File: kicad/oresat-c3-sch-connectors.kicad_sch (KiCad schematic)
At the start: 15 parts, among them J1 Conn_02x26_Odd_Even, J2 Conn_02x26_Odd_Even, J7 2-1734592-0

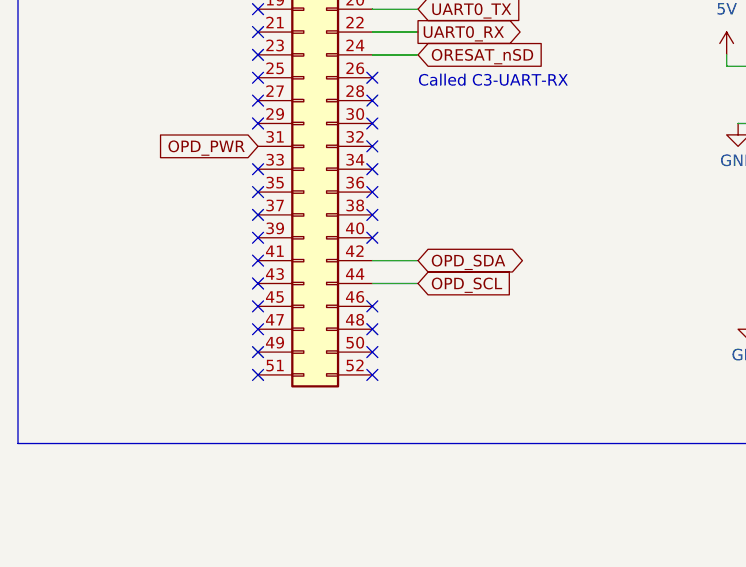
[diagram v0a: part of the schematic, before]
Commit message: Added I2C1 bus lines
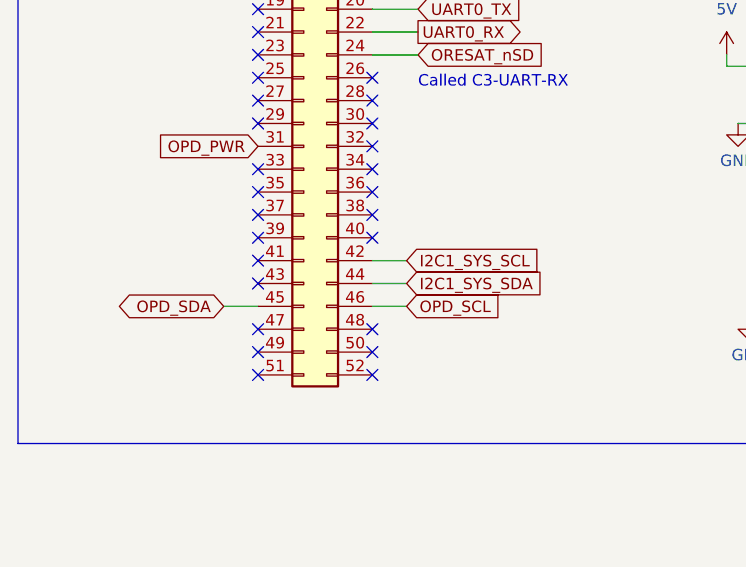
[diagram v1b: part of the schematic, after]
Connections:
- net OPD_SCL: now also J1.46 (Pin_46); no longer J1.44 (Pin_44)
- net OPD_SDA: now also J1.45 (Pin_45); no longer J1.42 (Pin_42)
- new net I2C1_SYS_SCL: J1.42 (Pin_42)
- new net I2C1_SYS_SDA: J1.44 (Pin_44)
- no-connect marks 92 -> 90
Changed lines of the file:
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@@
-	)
-	(no_connect
-		(at 113.03 113.03)
 	)
 	(no_connect
@@
 	)
 	(no_connect
-		(at 125.73 113.03)
-	)
-	(no_connect
 		(at 173.99 58.42)
 	)
@@
 	(wire
 		(pts
-			(xy 125.73 110.49) (xy 130.81 110.49)
-		)
-		(stroke
-			(width 0)
-			(type default)
-		)
-	)
-	(wire
-		(pts
 			(xy 275.59 101.6) (xy 273.05 101.6)
 		)
@@
 	(wire
 		(pts
-			(xy 125.73 107.95) (xy 130.81 107.95)
-		)
-		(stroke
-			(width 0)
-			(type default)
-		)
-	)
-	(wire
-		(pts
 			(xy 273.05 111.76) (xy 275.59 111.76)
 		)
@@
 	(wire
 		(pts
+			(xy 125.73 110.49) (xy 129.54 110.49)
+		)
+		(stroke
+			(width 0)
+			(type default)
+		)
+	)
+	(wire
+		(pts
 			(xy 262.89 130.81) (xy 262.89 134.62)
 		)
@@
 	(wire
 		(pts
+			(xy 125.73 113.03) (xy 129.54 113.03)
+		)
+		(stroke
+			(width 0)
+			(type default)
+		)
+	)
+	(wire
+		(pts
 			(xy 171.45 91.44) (xy 171.45 92.71)
 		)
@@
 	(wire
 		(pts
+			(xy 125.73 107.95) (xy 129.54 107.95)
+		)
+		(stroke
+			(width 0)
+			(type default)
+		)
+	)
+	(wire
+		(pts
 			(xy 166.37 92.71) (xy 171.45 92.71)
 		)
@@
 		(pts
 			(xy 167.64 114.3) (xy 173.99 114.3)
+		)
+		(stroke
+			(width 0)
+			(type default)
+		)
+	)
+	(wire
+		(pts
+			(xy 109.22 113.03) (xy 113.03 113.03)
 		)
 		(stroke
@@
 		)
 	)
+	(global_label "I2C1_SYS_SDA"
+		(shape input)
+		(at 129.54 110.49 0)
+		(fields_autoplaced yes)
+		(effects
+			(font
+				(size 1.27 1.27)
+			)
+			(justify left)
+		)
+		(property "Intersheetrefs" "${INTERSHEET_REFS}"
+			(at 145.8299 110.49 0)
+			(effects
+				(font
+					(size 1.27 1.27)
+				)
+				(justify left)
+			)
+		)
+	)
 	(global_label "OPD_SDA"
 		(shape bidirectional)
-		(at 130.81 107.95 0)
-		(fields_autoplaced yes)
-		(effects
-			(font
-				(size 1.27 1.27)
-			)
-			(justify left)
-		)
-		(property "Intersheetrefs" "${INTERSHEET_REFS}"
-			(at 143.3127 107.95 0)
-			(effects
-				(font
-					(size 1.27 1.27)
-				)
-				(justify left)
+		(at 109.22 113.03 180)
+		(fields_autoplaced yes)
+		(effects
+			(font
+				(size 1.27 1.27)
+			)
+			(justify right)
+		)
+		(property "Intersheetrefs" "${INTERSHEET_REFS}"
+			(at 96.7173 113.03 0)
+			(effects
+				(font
+					(size 1.27 1.27)
+				)
+				(justify right)
 			)
 		)
@@
 		)
 	)
+	(global_label "I2C1_SYS_SCL"
+		(shape input)
+		(at 129.54 107.95 0)
+		(fields_autoplaced yes)
+		(effects
+			(font
+				(size 1.27 1.27)
+			)
+			(justify left)
+		)
+		(property "Intersheetrefs" "${INTERSHEET_REFS}"
+			(at 145.7694 107.95 0)
+			(effects
+				(font
+					(size 1.27 1.27)
+				)
+				(justify left)
+			)
+		)
+	)
 	(global_label "USB_CLI_DM"
 		(shape bidirectional)
@@
 	(global_label "OPD_SCL"
 		(shape input)
-		(at 130.81 110.49 0)
-		(fields_autoplaced yes)
-		(effects
-			(font
-				(size 1.27 1.27)
-			)
-			(justify left)
-		)
-		(property "Intersheetrefs" "${INTERSHEET_REFS}"
-			(at 142.1409 110.49 0)
-			(effects
-				(font
+		(at 129.54 113.03 0)
+		(fields_autoplaced yes)
+		(effects
+			(font
+				(size 1.27 1.27)
+			)
+			(justify left)
+		)
+		(property "Intersheetrefs" "${INTERSHEET_REFS}"
+			(at 140.8709 113.03 0)
+			(effects
+				(font

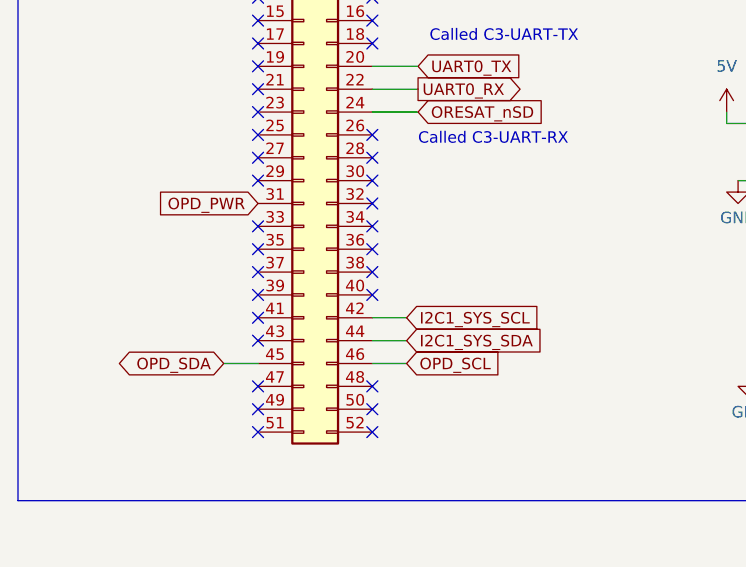
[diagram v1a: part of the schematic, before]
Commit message: Removed OPD and added LTC4300A to I2C1 bus
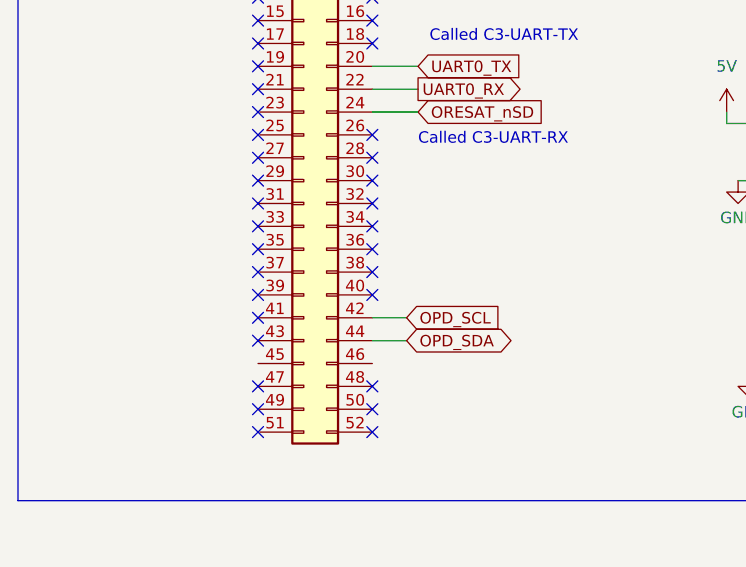
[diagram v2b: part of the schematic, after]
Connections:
- net I2C1_SYS_SCL is gone; now on net OPD_SCL: J1.42 (Pin_42)
- net I2C1_SYS_SDA is gone; now on net OPD_SDA: J1.44 (Pin_44)
- net OPD_SCL: no longer J1.46 (Pin_46)
- net OPD_SDA: no longer J1.45 (Pin_45)
- net OPD_PWR: no longer names the net of J1.31 (Pin_31)
- no-connect marks 90 -> 91
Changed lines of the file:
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@@
+	)
+	(no_connect
+		(at 113.03 95.25)
 	)
 	(no_connect
@@
 	(wire
 		(pts
+			(xy 262.89 130.81) (xy 262.89 134.62)
+		)
+		(stroke
+			(width 0)
+			(type default)
+		)
+	)
+	(wire
+		(pts
+			(xy 125.73 107.95) (xy 129.54 107.95)
+		)
+		(stroke
+			(width 0)
+			(type default)
+		)
+	)
+	(wire
+		(pts
+			(xy 274.32 130.81) (xy 262.89 130.81)
+		)
+		(stroke
+			(width 0)
+			(type default)
+		)
+	)
+	(wire
+		(pts
+			(xy 280.67 96.52) (xy 273.05 96.52)
+		)
+		(stroke
+			(width 0)
+			(type default)
+		)
+	)
+	(wire
+		(pts
+			(xy 279.4 73.66) (xy 280.67 73.66)
+		)
+		(stroke
+			(width 0)
+			(type default)
+		)
+	)
+	(wire
+		(pts
+			(xy 280.67 88.9) (xy 273.05 88.9)
+		)
+		(stroke
+			(width 0)
+			(type default)
+		)
+	)
+	(wire
+		(pts
 			(xy 125.73 110.49) (xy 129.54 110.49)
 		)
@@
 	(wire
 		(pts
-			(xy 262.89 130.81) (xy 262.89 134.62)
-		)
-		(stroke
-			(width 0)
-			(type default)
-		)
-	)
-	(wire
-		(pts
-			(xy 274.32 130.81) (xy 262.89 130.81)
-		)
-		(stroke
-			(width 0)
-			(type default)
-		)
-	)
-	(wire
-		(pts
-			(xy 280.67 96.52) (xy 273.05 96.52)
-		)
-		(stroke
-			(width 0)
-			(type default)
-		)
-	)
-	(wire
-		(pts
-			(xy 279.4 73.66) (xy 280.67 73.66)
-		)
-		(stroke
-			(width 0)
-			(type default)
-		)
-	)
-	(wire
-		(pts
-			(xy 280.67 88.9) (xy 273.05 88.9)
-		)
-		(stroke
-			(width 0)
-			(type default)
-		)
-	)
-	(wire
-		(pts
 			(xy 186.69 86.36) (xy 194.31 86.36)
 		)
@@
 	(wire
 		(pts
-			(xy 125.73 113.03) (xy 129.54 113.03)
-		)
-		(stroke
-			(width 0)
-			(type default)
-		)
-	)
-	(wire
-		(pts
 			(xy 171.45 91.44) (xy 171.45 92.71)
 		)
@@
 	(wire
 		(pts
-			(xy 125.73 107.95) (xy 129.54 107.95)
-		)
-		(stroke
-			(width 0)
-			(type default)
-		)
-	)
-	(wire
-		(pts
 			(xy 166.37 92.71) (xy 171.45 92.71)
 		)
@@
 		(pts
 			(xy 167.64 114.3) (xy 173.99 114.3)
-		)
-		(stroke
-			(width 0)
-			(type default)
-		)
-	)
-	(wire
-		(pts
-			(xy 109.22 113.03) (xy 113.03 113.03)
 		)
 		(stroke
@@
 		)
 	)
-	(global_label "I2C1_SYS_SDA"
-		(shape input)
-		(at 129.54 110.49 0)
-		(fields_autoplaced yes)
-		(effects
-			(font
-				(size 1.27 1.27)
-			)
-			(justify left)
-		)
-		(property "Intersheetrefs" "${INTERSHEET_REFS}"
-			(at 145.8299 110.49 0)
-			(effects
-				(font
-					(size 1.27 1.27)
-				)
-				(justify left)
-			)
-		)
-	)
 	(global_label "OPD_SDA"
 		(shape bidirectional)
-		(at 109.22 113.03 180)
-		(fields_autoplaced yes)
-		(effects
-			(font
-				(size 1.27 1.27)
-			)
-			(justify right)
-		)
-		(property "Intersheetrefs" "${INTERSHEET_REFS}"
-			(at 96.7173 113.03 0)
-			(effects
-				(font
-					(size 1.27 1.27)
-				)
-				(justify right)
+		(at 129.54 110.49 0)
+		(fields_autoplaced yes)
+		(effects
+			(font
+				(size 1.27 1.27)
+			)
+			(justify left)
+		)
+		(property "Intersheetrefs" "${INTERSHEET_REFS}"
+			(at 142.0427 110.49 0)
+			(effects
+				(font
+					(size 1.27 1.27)
+				)
+				(justify left)
 			)
 		)
@@
 		)
 	)
-	(global_label "OPD_PWR"
-		(shape input)
-		(at 113.03 95.25 180)
-		(fields_autoplaced yes)
-		(effects
-			(font
-				(size 1.27 1.27)
-			)
-			(justify right)
-		)
-		(property "Intersheetrefs" "${INTERSHEET_REFS}"
-			(at 101.2153 95.25 0)
-			(effects
-				(font
-					(size 1.27 1.27)
-				)
-				(justify right)
-			)
-		)
-	)
 	(global_label "CAN1L-"
 		(shape input)
@@
 		)
 	)
-	(global_label "I2C1_SYS_SCL"
-		(shape input)
-		(at 129.54 107.95 0)
-		(fields_autoplaced yes)
-		(effects
-			(font
-				(size 1.27 1.27)
-			)
-			(justify left)
-		)
-		(property "Intersheetrefs" "${INTERSHEET_REFS}"
-			(at 145.7694 107.95 0)
-			(effects
-				(font
-					(size 1.27 1.27)
-				)
-				(justify left)
-			)
-		)
-	)
 	(global_label "USB_CLI_DM"
 		(shape bidirectional)
@@
 	(global_label "OPD_SCL"
 		(shape input)
-		(at 129.54 113.03 0)
-		(fields_autoplaced yes)
-		(effects
-			(font
-				(size 1.27 1.27)
-			)
-			(justify left)
-		)
-		(property "Intersheetrefs" "${INTERSHEET_REFS}"
-			(at 140.8709 113.03 0)
-			(effects
-				(font
+		(at 129.54 107.95 0)
+		(fields_autoplaced yes)
+		(effects
+			(font
+				(size 1.27 1.27)
+			)
+			(justify left)
+		)
+		(property "Intersheetrefs" "${INTERSHEET_REFS}"
+			(at 140.8709 107.95 0)
+			(effects
+				(font

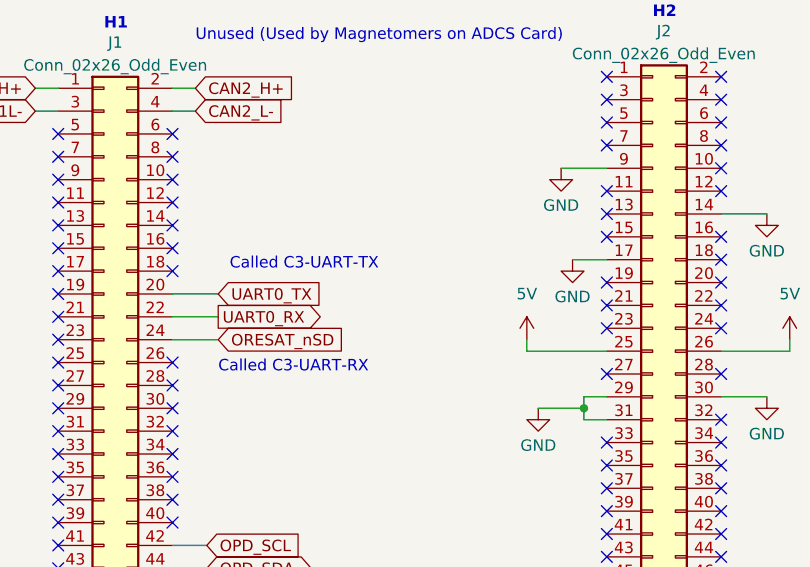
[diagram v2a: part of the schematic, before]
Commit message: Added GPIO enable pins for ADCS
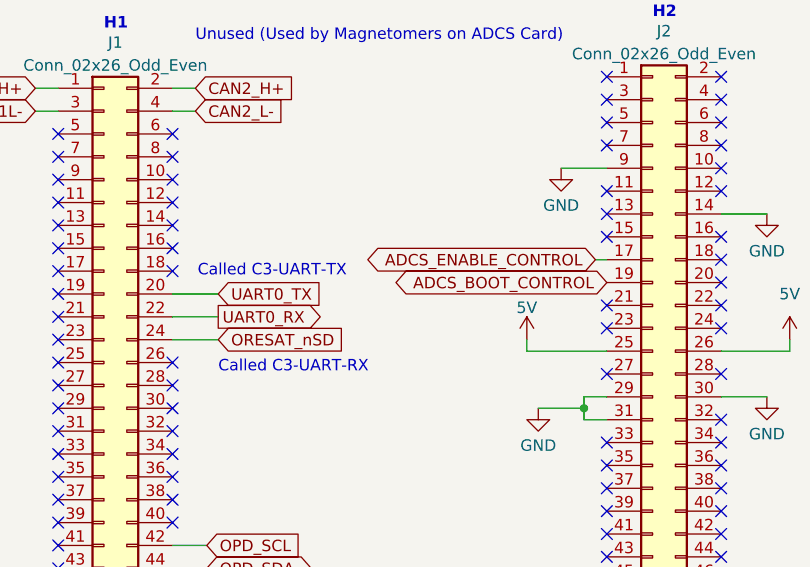
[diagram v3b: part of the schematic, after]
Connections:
- net GND: no longer J2.17 (Pin_17)
- net ADCS_BOOT_CONTROL: now reaches J2.19 (Pin_19)
- new net ADCS_ENABLE_CONTROL: J2.17 (Pin_17)
- no-connect marks 91 -> 90
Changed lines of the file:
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@@
-	)
-	(no_connect
-		(at 173.99 78.74)
 	)
 	(no_connect
@@
 	(wire
 		(pts
+			(xy 172.72 76.2) (xy 173.99 76.2)
+		)
+		(stroke
+			(width 0)
+			(type default)
+		)
+	)
+	(wire
+		(pts
 			(xy 130.81 80.01) (xy 125.73 80.01)
 		)
@@
 		(pts
 			(xy 273.05 114.3) (xy 275.59 114.3)
-		)
-		(stroke
-			(width 0)
-			(type default)
-		)
-	)
-	(wire
-		(pts
-			(xy 170.18 76.2) (xy 173.99 76.2)
 		)
 		(stroke
@@
 	(text "Called C3-UART-TX"
 		(exclude_from_sim no)
-		(at 132.08 77.47 0)
+		(at 128.524 78.232 0)
 		(effects
 			(font
@@
 		)
 	)
+	(global_label "ADCS_BOOT_CONTROL"
+		(shape bidirectional)
+		(at 173.99 78.74 180)
+		(fields_autoplaced yes)
+		(effects
+			(font
+				(size 1.27 1.27)
+			)
+			(justify right)
+		)
+		(property "Intersheetrefs" "${INTERSHEET_REFS}"
+			(at 149.6944 78.74 0)
+			(effects
+				(font
+					(size 1.27 1.27)
+				)
+				(justify right)
+			)
+		)
+	)
 	(global_label "CAN1L-"
 		(shape input)
@@
 		(property "Intersheetrefs" "${INTERSHEET_REFS}"
 			(at 100.0057 59.69 0)
+			(effects
+				(font
+					(size 1.27 1.27)
+				)
+				(justify right)
+			)
+		)
+	)
+	(global_label "ADCS_ENABLE_CONTROL"
+		(shape bidirectional)
+		(at 172.72 76.2 180)
+		(fields_autoplaced yes)
+		(effects
+			(font
+				(size 1.27 1.27)
+			)
+			(justify right)
+		)
+		(property "Intersheetrefs" "${INTERSHEET_REFS}"
+			(at 146.3078 76.2 0)
 			(effects
 				(font
@@
 		(on_board yes)
 		(dnp no)
-		(fields_autoplaced yes)
 		(property "Reference" "#5V01"
 			(at 165.1 88.9 0)
@@
 		)
 		(property "Value" "5V"
-			(at 165.1 80.01 0)
+			(at 165.1 81.534 0)
 			(effects
 				(font
@@
 					(unit 1)
 				)
-			)
-		)
-	)
-	(symbol
-		(lib_id "power:GND")
-		(at 170.18 76.2 0)
-		(unit 1)
-		(exclude_from_sim no)
-		(in_bom yes)
-		(on_board yes)
-		(dnp no)
-		(fields_autoplaced yes)
-		(property "Reference" "#PWR021"
-			(at 170.18 82.55 0)
-			(effects
-				(font
-					(size 1.27 1.27)
-				)
-				(hide yes)
-			)
-		)
-		(property "Value" "GND"
-			(at 170.18 80.3355 0)
-			(effects
-				(font
-					(size 1.27 1.27)
-				)
-			)
-		)
-		(property "Footprint" ""
-			(at 170.18 76.2 0)
-			(effects
-				(font
-					(size 1.27 1.27)
-				)
-				(hide yes)
-			)
-		)
-		(property "Datasheet" ""
-			(at 170.18 76.2 0)
-			(effects
-				(font
-					(size 1.27 1.27)
-				)
-				(hide yes)
-			)
-		)
-		(property "Description" ""
-			(at 170.18 76.2 0)
-			(effects
-				(font
-					(size 1.27 1.27)
-				)
-				(hide yes)
-			)
-		)
-		(pin "1"
-		)
-		(instances
-			(project "oresat-c3"
-				(path "/65d12cdd-c326-4033-9053-c59fa4e0b25e/b9a61b98-fba0-4063-a603-e7fc9d7070a0"
-					(reference "#PWR021")
-					(unit 1)
-				)
